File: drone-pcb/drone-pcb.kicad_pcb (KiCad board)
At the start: 2 copper layers, 60 x 27.5 mm, 37 parts, among them J1 Conn_02x01, J2 Conn_02x01, J3 Conn_02x01, J4 Conn_02x01, J5 Conn_02x01, Q1 NMOS, Q2 NMOS, Q3 NMOS, Q4 NMOS, Q5 NPN, Q6 NPN, U1 XIAO-MG24-DIP

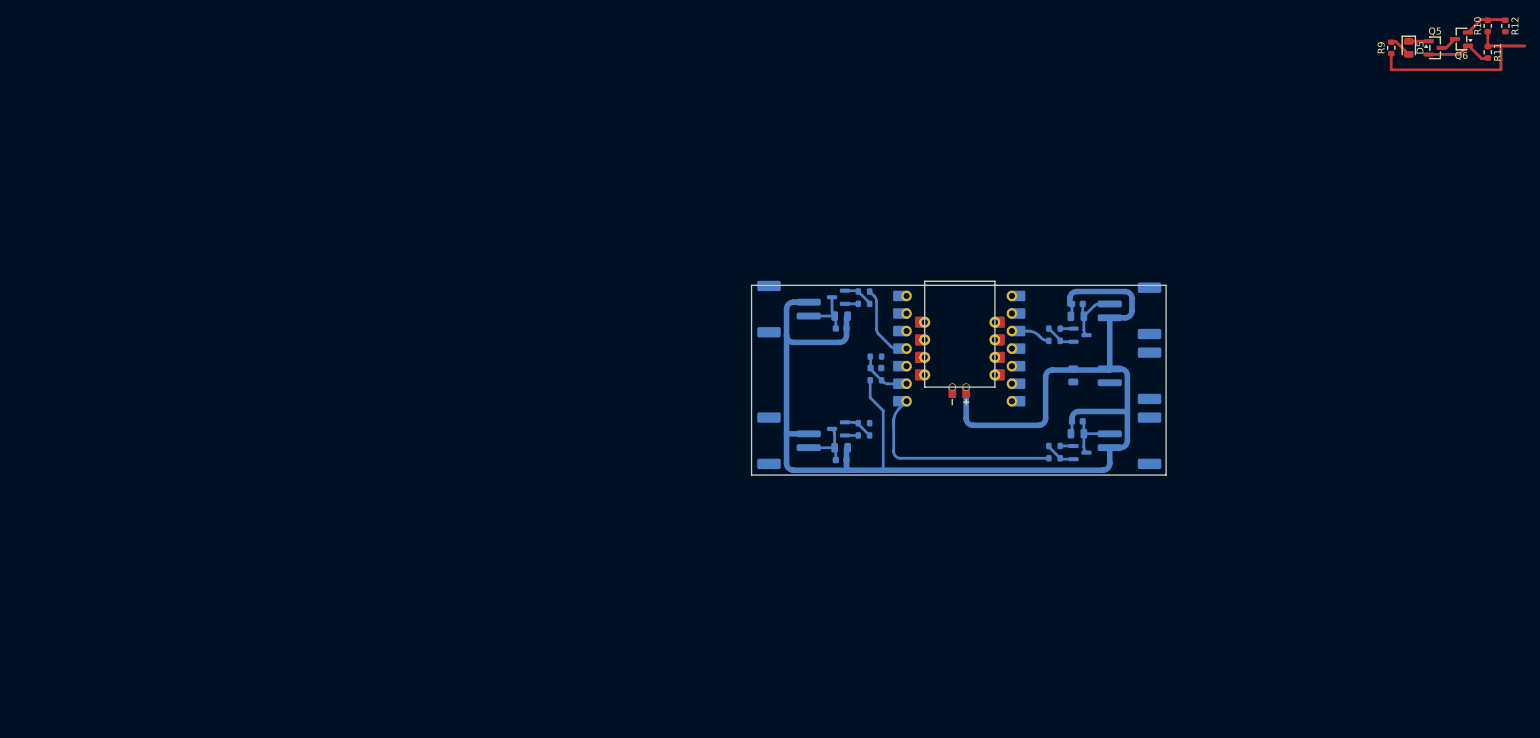
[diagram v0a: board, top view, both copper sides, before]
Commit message: apdejt rev 2
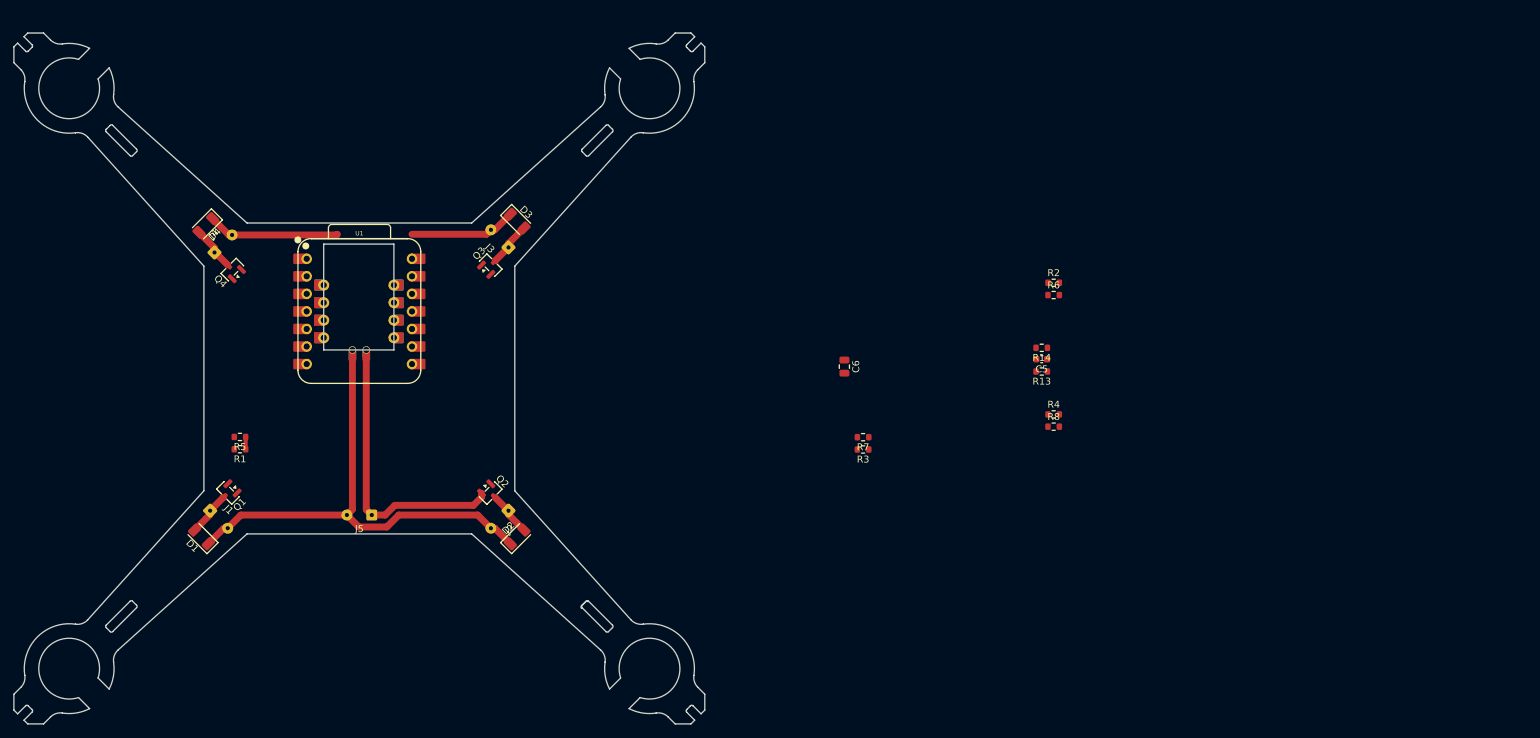
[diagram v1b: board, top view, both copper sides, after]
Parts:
- removed C1, C2, C3, C4: 0.1u, Capacitor_SMD:C_0603_1608Metric
- removed D5: LXZ1-PL02, Diode_SMD:D_0805_2012Metric
- removed Q5, Q6: NPN, Package_TO_SOT_SMD:SOT-23
- removed R10: 39k, Resistor_SMD:R_0603_1608Metric
- removed R11, R12: 10k, Resistor_SMD:R_0603_1608Metric
- removed R9: 100, Resistor_SMD:R_0603_1608Metric
- C5, C6, R1, R13, R14, R2, R4, R5, R6, R8: moved to F.Cu
- D1, D2, D3, D4: value 1N5819 -> SD1206T040S2R0; footprint Diode_SMD:D_0805_2012Metric -> Diode_SMD:D_1206_3216Metric; moved to F.Cu
- J1: value Conn_02x01 -> MOT_1; footprint Connector_JST:JST_PH_S2B-PH-SM4-TB_1x02-1MP_P2.00mm_Horizontal -> Connector_Wire:SolderWire-0.1sqmm_1x02_P3.6mm_D0.4mm_OD1mm; moved to F.Cu
- J2: value Conn_02x01 -> MOT_2; footprint Connector_JST:JST_PH_S2B-PH-SM4-TB_1x02-1MP_P2.00mm_Horizontal -> Connector_Wire:SolderWire-0.1sqmm_1x02_P3.6mm_D0.4mm_OD1mm; moved to F.Cu
- J3: value Conn_02x01 -> MOT_3; footprint Connector_JST:JST_PH_S2B-PH-SM4-TB_1x02-1MP_P2.00mm_Horizontal -> Connector_Wire:SolderWire-0.1sqmm_1x02_P3.6mm_D0.4mm_OD1mm; moved to F.Cu
- J4: value Conn_02x01 -> MOT_4; footprint Connector_JST:JST_PH_S2B-PH-SM4-TB_1x02-1MP_P2.00mm_Horizontal -> Connector_Wire:SolderWire-0.1sqmm_1x02_P3.6mm_D0.4mm_OD1mm; moved to F.Cu
- J5: value Conn_02x01 -> BAT; footprint Connector_JST:JST_PH_S2B-PH-SM4-TB_1x02-1MP_P2.00mm_Horizontal -> Connector_Wire:SolderWire-0.1sqmm_1x02_P3.6mm_D0.4mm_OD1mm; moved to F.Cu
- Q1, Q2, Q3, Q4: value NMOS -> AO3400A; moved to F.Cu
- R3: value 100 -> 10k; moved to F.Cu
- R7: value 10k -> 100; moved to F.Cu
- U1: value XIAO-MG24-DIP -> XIAO ESP32C3; moved to F.Cu
- moved J1 136.2 mm to (94.5, 91.0), turned to -45 degrees
- moved D1 130.8 mm to (93.2, 94.9), turned to 135 degrees
- moved Q1 125.4 mm to (97.1, 88.5), turned to -135 degrees
- moved R1 118.9 mm to (98.8, 82.2), turned to 180 degrees
- moved R5 118.9 mm to (98.8, 80.4), turned to 180 degrees
- moved J5 111.5 mm to (117.9, 91.7), turned to 180 degrees
- moved D4 97.4 mm to (93.9, 49.8), turned to -135 degrees
- moved J3 94.1 mm to (137.7, 52.9), turned to 135 degrees
- moved Q4 90.7 mm to (97.7, 56.2), turned to 135 degrees
- moved Q3 89.5 mm to (135.1, 55.5), turned to 45 degrees
- moved J4 87.5 mm to (95.2, 53.7), turned to 45 degrees
- moved U1 87.0 mm to (116.1, 62.2)
- moved D3 86.7 mm to (139.0, 49.1), turned to -45 degrees
- moved Q2 57.8 mm to (135.1, 88.5), turned to -45 degrees
- moved D2 56.7 mm to (139.0, 94.9), turned to 45 degrees
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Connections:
- net V_MOT1- renamed Net-(D1-A)
- net V_MOT2- renamed Net-(D2-A)
- net V_MOT3- renamed Net-(D3-A)
- net V_MOT4- renamed Net-(D4-A)
- C5 pad 1: Net-(U1-PA03_A8_D8_SCK) -> BAT_SENS
- J5 pad 1: V_BAT -> GND
- J5 pad 2: GND -> V_BAT
- R1 pad 1: Motor_1 -> MOT_1
- R13 pad 2: Net-(U1-PA03_A8_D8_SCK) -> BAT_SENS
- R14 pad 1: Net-(U1-PA03_A8_D8_SCK) -> BAT_SENS
- R2 pad 1: Motor_2 -> MOT_2
- R3 pad 1: Motor_3 -> MOT_2
- R3 pad 2: Net-(Q3-G) -> GND
- R4 pad 1: Motor_4 -> MOT_3
- R4 pad 2: Net-(Q4-G) -> Net-(Q3-G)
- R5 pad 1: Net-(Q1-G) -> MOT_1
- R6 pad 1: Net-(Q2-G) -> MOT_3
- R7 pad 1: Net-(Q3-G) -> MOT_4
- R7 pad 2: GND -> Net-(Q4-G)
- R8 pad 1: Net-(Q4-G) -> MOT_4
- U1 pad 10: Motor_4 -> unconnected-(U1-D9-Pad10)
- U1 pad 11: Motor_2 -> unconnected-(U1-D10-Pad11)
- U1 pad 13: GND -> unconnected-(U1-GND-Pad13)
- U1 pad 3: Motor_1 -> unconnected-(U1-D2-Pad3)
- U1 pad 8: Motor_3 -> unconnected-(U1-D7-Pad8)
- U1 pad 9: Net-(U1-PA03_A8_D8_SCK) -> unconnected-(U1-D8-Pad9)
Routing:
- net V_BAT: track 223.1 -> 106.4 mm
- net GND: track 7.69 -> 40.8 mm
- net Motor_3: track 31.7 -> 0.00 mm
- net Motor_2: track 10.7 -> 0.00 mm
- net Net-(Q5-B): track 9.89 -> 0.00 mm
- net Net-(U1-PA03_A8_D8_SCK): track 7.13 -> 0.00 mm
- net Net-(Q6-B): track 6.19 -> 0.00 mm
- net Motor_1: track 4.97 -> 0.00 mm
- net Net-(Q3-G): track 4.43 -> 0.00 mm
- net Net-(Q1-G): track 4.43 -> 0.00 mm
- net Net-(Q2-G): track 4.43 -> 0.00 mm
- net Net-(Q4-G): track 4.31 -> 0.00 mm
- net Net-(D5-A): track 3.34 -> 0.00 mm
- net Net-(D5-K): track 2.88 -> 0.00 mm
- net Net-(D1-A): track 9.20 -> 6.45 mm
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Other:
- board size 60 x 27.5 mm -> 100 x 100 mm
